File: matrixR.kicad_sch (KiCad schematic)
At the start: 68 parts

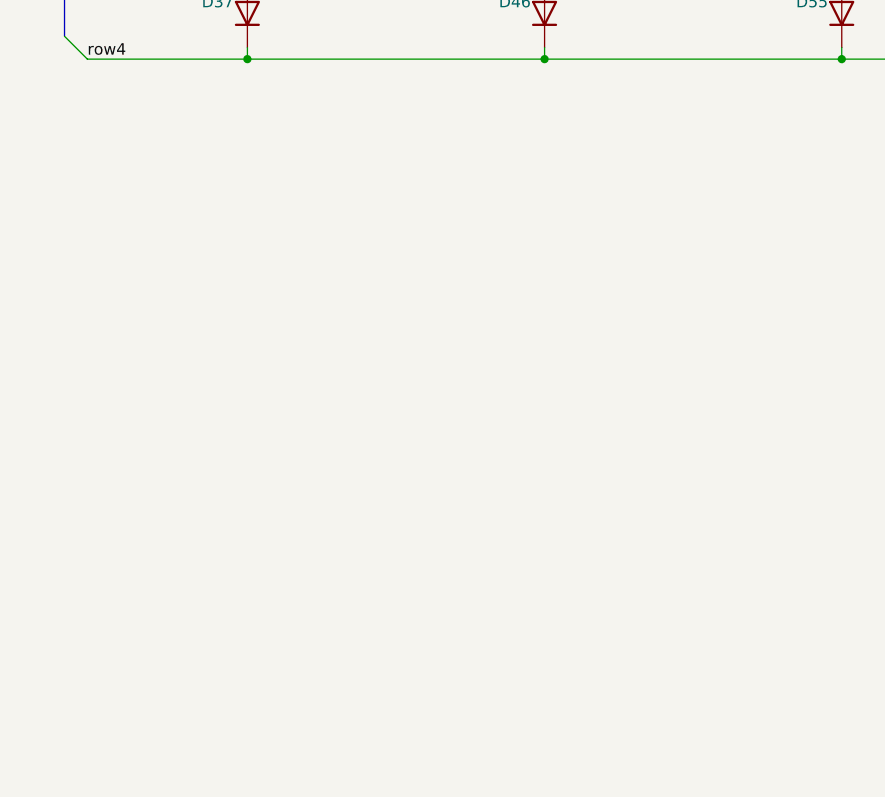
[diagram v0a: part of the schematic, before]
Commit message: plates added
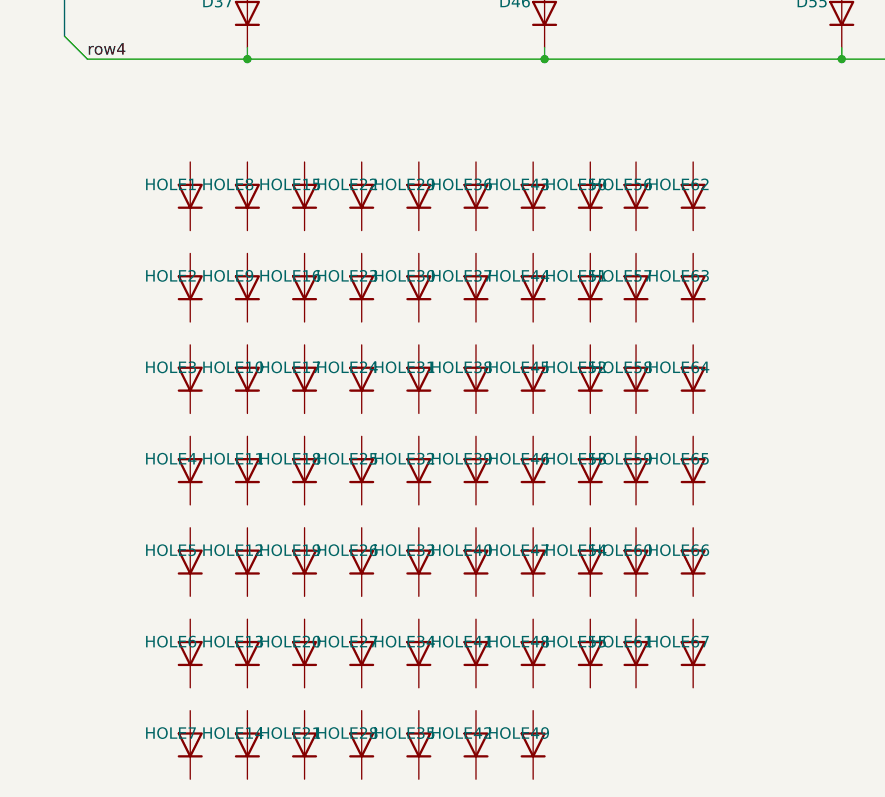
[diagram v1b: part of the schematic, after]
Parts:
- added HOLE1, HOLE10, HOLE11, HOLE12, HOLE13, HOLE14, HOLE15, HOLE16, HOLE17, HOLE18, HOLE19, HOLE2, HOLE20, HOLE21, HOLE22, HOLE23, HOLE24, HOLE25, HOLE26, HOLE27, HOLE28, HOLE29, HOLE3, HOLE30, HOLE31, HOLE32, HOLE33, HOLE34, HOLE35, HOLE36, HOLE37, HOLE38, HOLE39, HOLE4, HOLE40, HOLE41, HOLE42, HOLE43, HOLE44, HOLE45, HOLE46, HOLE47, HOLE48, HOLE49, HOLE5, HOLE50, HOLE51, HOLE52, HOLE53, HOLE54, HOLE55, HOLE56, HOLE57, HOLE58, HOLE59, HOLE6, HOLE60, HOLE61, HOLE62, HOLE63, HOLE64, HOLE65, HOLE66, HOLE67, HOLE7, HOLE8, HOLE9: ~, arisu-split:plate_hole, symbol Device:D
